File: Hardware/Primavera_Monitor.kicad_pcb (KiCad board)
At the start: 2 copper layers, 67.3 x 96.5 mm, 20 parts, among them J1 Conn_01x02, U1 OPB720b_mod, U2 SD_Card_Interface, U3 BackBoard, U4 RTC_DS3231_Mod, U5 IFX27001TFV33, U6 BME280_Mod_LC, U7 MPU6050_Mod, U8 MPU6050_Mod

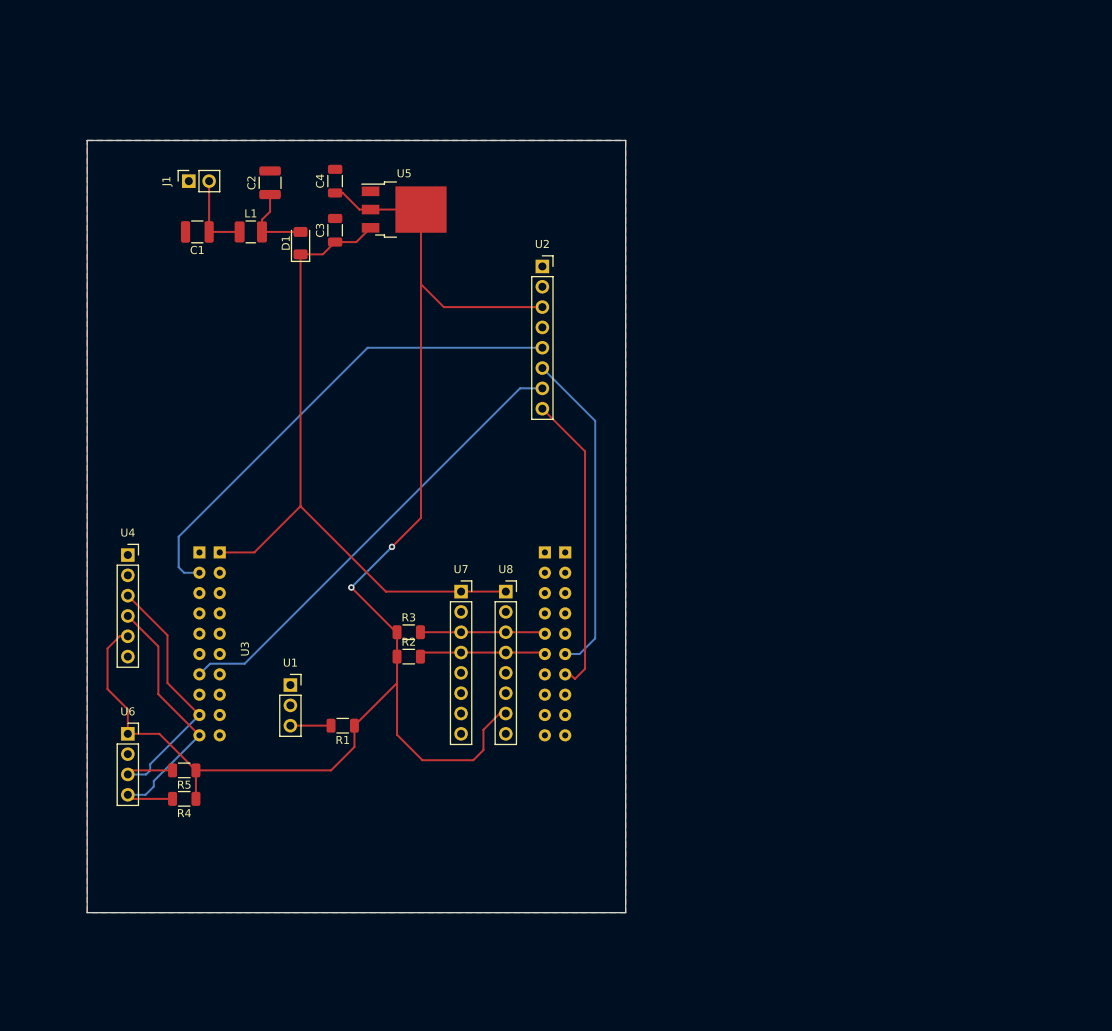
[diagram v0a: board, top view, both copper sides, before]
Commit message: Add PCB design
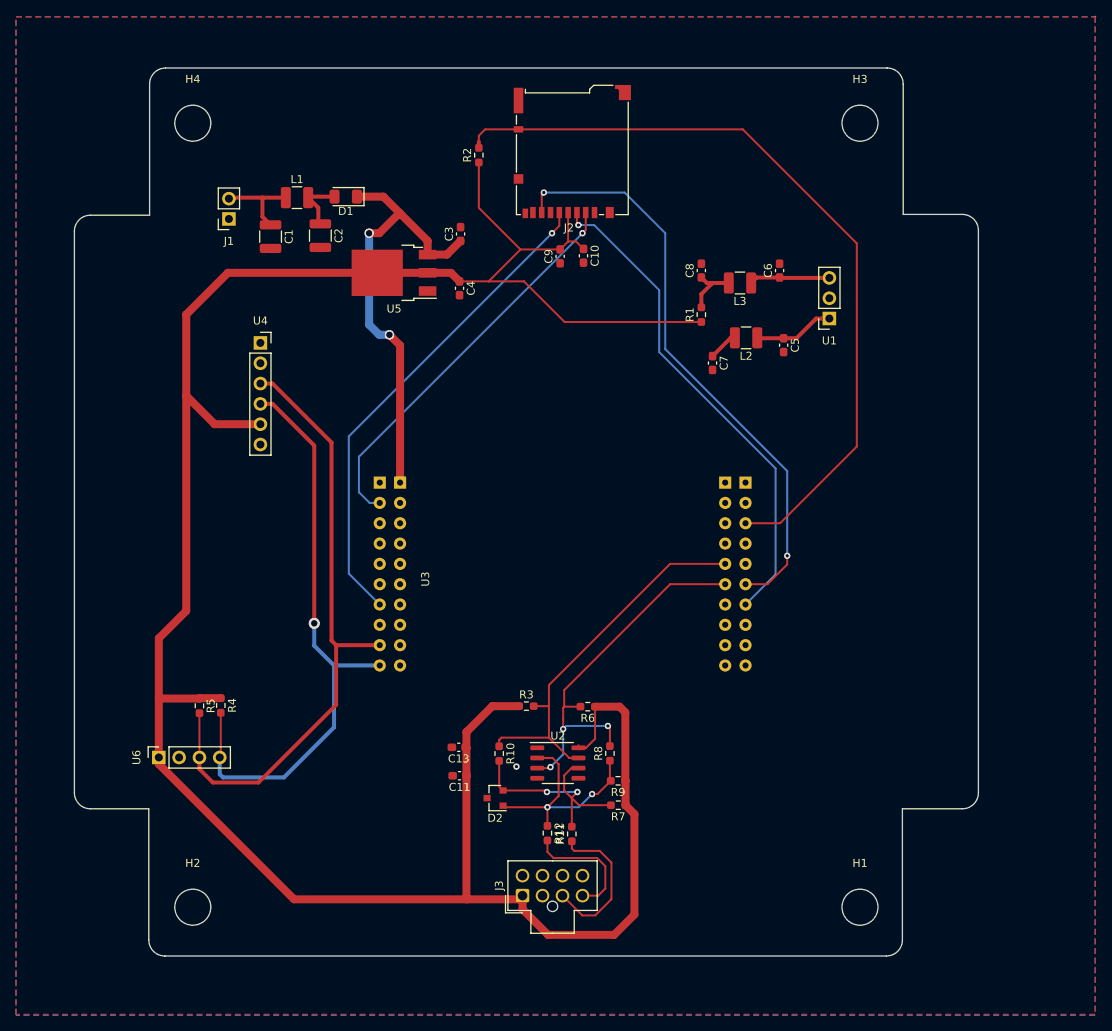
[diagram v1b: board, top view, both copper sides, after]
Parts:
- removed U7, U8: MPU6050_Mod, Connector_PinSocket_2.54mm:PinSocket_1x08_P2.54mm_Vertical
- added C10: C, Capacitor_SMD:C_0603_1608Metric_Pad1.08x0.95mm_HandSolder, F.Cu at (125.5, 62.7)
- added C11: C, Capacitor_SMD:C_0603_1608Metric_Pad1.08x0.95mm_HandSolder, F.Cu at (110.0, 127.7)
- added C13: C, Capacitor_SMD:C_0603_1608Metric_Pad1.08x0.95mm_HandSolder, F.Cu at (109.9, 124.1)
- added C5: C, Capacitor_SMD:C_0603_1608Metric_Pad1.08x0.95mm_HandSolder, F.Cu at (150.6, 73.8)
- added C6: C, Capacitor_SMD:C_0603_1608Metric_Pad1.08x0.95mm_HandSolder, F.Cu at (150.0, 64.5)
- added C7: C, Capacitor_SMD:C_0603_1608Metric_Pad1.08x0.95mm_HandSolder, F.Cu at (141.7, 76.1)
- added C8: C, Capacitor_SMD:C_0603_1608Metric_Pad1.08x0.95mm_HandSolder, F.Cu at (140.3, 64.5)
- added C9: C, Capacitor_SMD:C_0603_1608Metric_Pad1.08x0.95mm_HandSolder, F.Cu at (122.6, 62.7)
- added D2: SP0502BAHT, Package_TO_SOT_SMD:SOT-23, F.Cu at (114.5, 130.5)
- added H1: MountingHole, MountingHole:MountingHole_4.5mm, F.Cu at (160.1, 144.1)
- added H2: MountingHole, MountingHole:MountingHole_4.5mm, F.Cu at (76.7, 144.1)
- added H3: MountingHole, MountingHole:MountingHole_4.5mm, F.Cu at (160.1, 46.1)
- added H4: MountingHole, MountingHole:MountingHole_4.5mm, F.Cu at (76.7, 46.1)
- added J2: Micro_SD_Card_Det, Connector_Card:microSD_HC_Hirose_DM3BT-DSF-PEJS, F.Cu at (124.1, 49.6)
- added J3: Conn_01x08, Connector_Molex:Molex_Nano-Fit_105310-xx08_2x04_P2.50mm_Vertical, F.Cu at (117.9, 142.7)
- added L2: L, Inductor_SMD:L_1210_3225Metric, F.Cu at (145.9, 72.9)
- added L3: L, Inductor_SMD:L_1210_3225Metric, F.Cu at (145.1, 66.1)
- added R10: R, Resistor_SMD:R_0603_1608Metric_Pad0.98x0.95mm_HandSolder, F.Cu at (115.0, 124.9)
- added R11: R, Resistor_SMD:R_0603_1608Metric_Pad0.98x0.95mm_HandSolder, F.Cu at (124.1, 134.9)
- added R12: R, Resistor_SMD:R_0603_1608Metric_Pad0.98x0.95mm_HandSolder, F.Cu at (121.0, 134.8)
- added R6: R, Resistor_SMD:R_0603_1608Metric_Pad0.98x0.95mm_HandSolder, F.Cu at (126.1, 119.0)
- added R7: R, Resistor_SMD:R_0603_1608Metric_Pad0.98x0.95mm_HandSolder, F.Cu at (129.9, 131.4)
- added R8: R, Resistor_SMD:R_0603_1608Metric_Pad0.98x0.95mm_HandSolder, F.Cu at (128.8, 124.9)
- added R9: R, Resistor_SMD:R_0603_1608Metric_Pad0.98x0.95mm_HandSolder, F.Cu at (129.9, 128.3)
- C3, C4: footprint Capacitor_SMD:C_1206_3216Metric -> Capacitor_SMD:C_0603_1608Metric_Pad1.08x0.95mm_HandSolder
- R1, R2, R3, R4, R5: footprint Resistor_SMD:R_1206_3216Metric -> Resistor_SMD:R_0603_1608Metric_Pad0.98x0.95mm_HandSolder
- U2: value SD_Card_Interface -> P82B715; footprint Connector_PinSocket_2.54mm:PinSocket_1x08_P2.54mm_Vertical -> Package_SO:SO-8_3.9x4.9mm_P1.27mm
- moved U1 81.5 mm to (156.3, 70.5), turned to 180 degrees
- moved R1 68.2 mm to (140.3, 70.0), turned to 90 degrees
- moved R2 63.3 mm to (112.5, 50.1), turned to 90 degrees
- moved U2 62.1 mm to (122.3, 126.1)
- moved U4 31.3 mm to (85.2, 73.6)
- moved U3 24.2 mm to (121.7, 102.5)
- moved C4 20.5 mm to (110.0, 66.7), turned to 270 degrees
- moved R3 17.4 mm to (118.4, 119.0)
- moved C3 15.7 mm to (110.2, 60.0)
- moved R4 12.5 mm to (80.2, 118.9), turned to 270 degrees
- moved C1 9.17 mm to (86.4, 60.3), turned to 270 degrees
- moved C2 9.12 mm to (92.6, 60.2), turned to 270 degrees
- moved R5 8.29 mm to (77.5, 118.9), turned to 270 degrees
- moved D1 8.10 mm to (95.8, 55.3), turned to 180 degrees
- moved U5 8.01 mm to (101.9, 64.8), turned to 180 degrees
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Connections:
- R2 pad 2: I2C_2_SDA -> SD_DET
- U1 pad 1: PWM -> Net-(C5-Pad1)
- U1 pad 3: CCR -> Net-(C6-Pad1)
- U2 pad 1: GND -> Net-(U2-Pad1)
- U2 pad 2: GND -> Net-(D2-Pad1)
- U2 pad 3: +3V3 -> I2C_2_SDA
- U2 pad 4: Net-(U2-Pad4) -> GND
- U2 pad 5: SPI_CS -> Net-(U2-Pad1)
- U2 pad 6: SPI_Tx -> Net-(D2-Pad2)
- U2 pad 7: SPI_CLK -> I2C_2_SCL
- U2 pad 8: SPI_Rx -> +3V3
- U3 pad 1: Net-(U3-Pad1) -> (no net)
- U3 pad 13: Net-(U3-Pad13) -> (no net)
- U3 pad 14: Net-(U3-Pad14) -> (no net)
- U3 pad 15: Net-(U3-Pad15) -> (no net)
- U3 pad 16: Net-(U3-Pad16) -> (no net)
- U3 pad 17: Net-(U3-Pad17) -> (no net)
- U3 pad 18: Net-(U3-Pad18) -> (no net)
- U3 pad 19: Net-(U3-Pad19) -> (no net)
- U3 pad 20: Net-(U3-Pad20) -> (no net)
- U3 pad 22: Net-(U3-Pad22) -> (no net)
- U3 pad 23: Net-(U3-Pad23) -> SD_DET
- U3 pad 24: Net-(U3-Pad24) -> (no net)
- U3 pad 25: Net-(U3-Pad25) -> (no net)
- U3 pad 28: Net-(U3-Pad28) -> (no net)
- U3 pad 29: Net-(U3-Pad29) -> (no net)
- U3 pad 3: Net-(U3-Pad3) -> (no net)
- U3 pad 30: Net-(U3-Pad30) -> (no net)
- U3 pad 31: Net-(U3-Pad31) -> (no net)
- U3 pad 32: Net-(U3-Pad32) -> (no net)
- U3 pad 33: Net-(U3-Pad33) -> (no net)
- U3 pad 34: Net-(U3-Pad34) -> (no net)
- U3 pad 37: Net-(U3-Pad37) -> (no net)
- U3 pad 38: Net-(U3-Pad38) -> (no net)
- U3 pad 39: Net-(U3-Pad39) -> (no net)
- U3 pad 4: Net-(U3-Pad4) -> (no net)
- U3 pad 40: Net-(U3-Pad40) -> (no net)
- U3 pad 5: Net-(U3-Pad5) -> (no net)
- U3 pad 6: Net-(U3-Pad6) -> (no net)
- U3 pad 8: Net-(U3-Pad8) -> (no net)
- U4 pad 1: Net-(U4-Pad1) -> (no net)
- U4 pad 2: Net-(U4-Pad2) -> (no net)
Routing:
- net +3V3: track 178.5 -> 312.6 mm, vias 2 -> 0
- net SD_DET: track 0.00 -> 98.3 mm
- net I2C_1_SCL: track 36.9 -> 79.2 mm
- net I2C_1_SDA: track 36.9 -> 75.6 mm, vias 0 -> 1
- net I2C_2_SCL: track 15.6 -> 48.7 mm
- net SPI_Tx: track 41.1 -> 73.8 mm, vias 0 -> 2
- net I2C_2_SDA: track 15.8 -> 48.0 mm, vias 0 -> 3
- net Net-(D2-Pad1): track 0.00 -> 28.7 mm, vias 0 -> 2
- net Net-(D2-Pad2): track 0.00 -> 28.5 mm, vias 0 -> 2
- net +5V: track 84.2 -> 56.0 mm, vias 0 -> 2
- net SPI_Rx: track 38.0 -> 62.0 mm, vias 0 -> 1
- net Net-(J3-Pad3): track 0.00 -> 19.1 mm
- net Net-(J3-Pad4): track 0.00 -> 15.4 mm
- net SPI_CS: track 61.9 -> 49.9 mm, vias 0 -> 1
- net Net-(C6-Pad1): track 0.00 -> 10.1 mm
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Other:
- board size 67.3 x 96.5 mm -> 113 x 111 mm
- board text added: "Enclosure: ELBE 12212085 SW"
